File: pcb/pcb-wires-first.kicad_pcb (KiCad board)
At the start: 2 copper layers, 93.7 x 67 mm, 50 parts, among them J10 Conn_01x02, J11 Conn_01x02, J2 Conn_01x02, J5 Conn_01x04, J6 Conn_01x04, J7 Conn_01x04, J9 Conn_01x02, SW1 off-2, SW2 on-2, SW3 on-1, SW4 off-1, SW5 on-3, SW6 off-3, U1 SLG47115V, U2 SLG46826V, U3 R-78C3.3-1.0

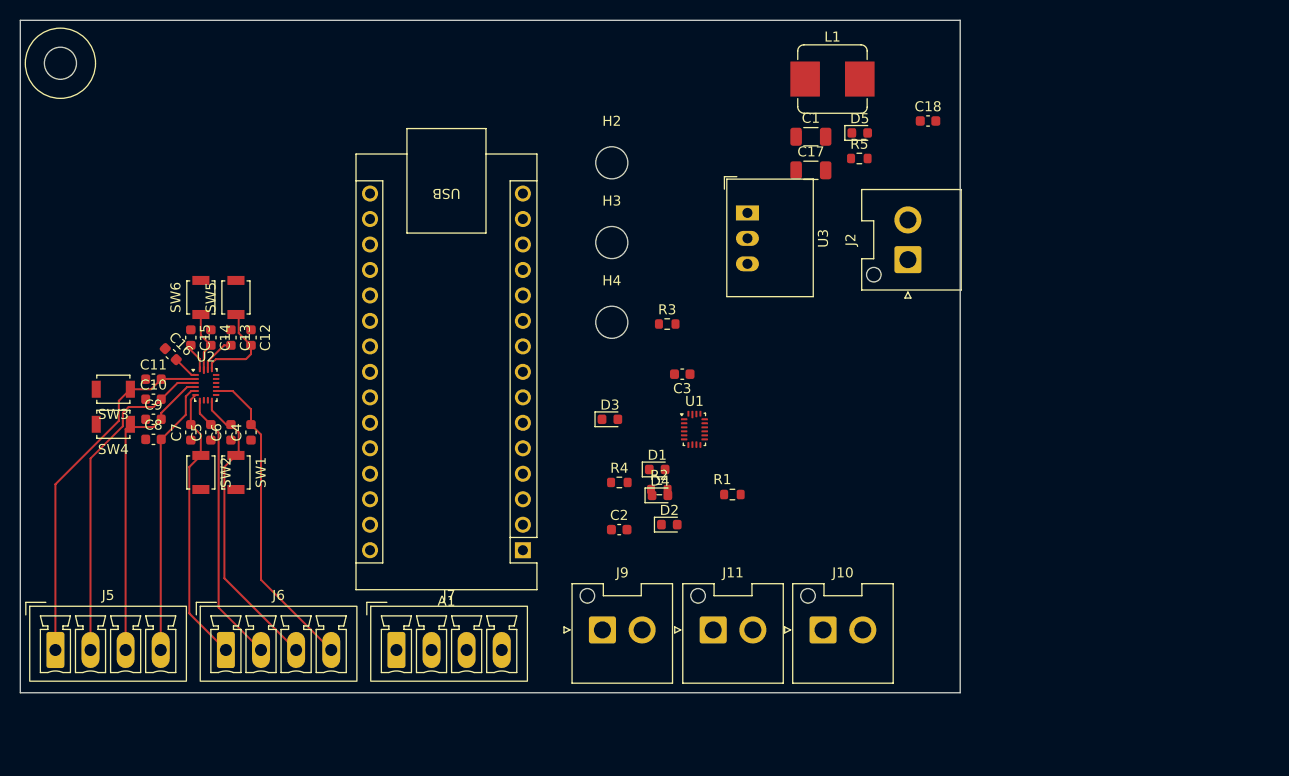
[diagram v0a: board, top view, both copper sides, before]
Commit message: Routing the board.
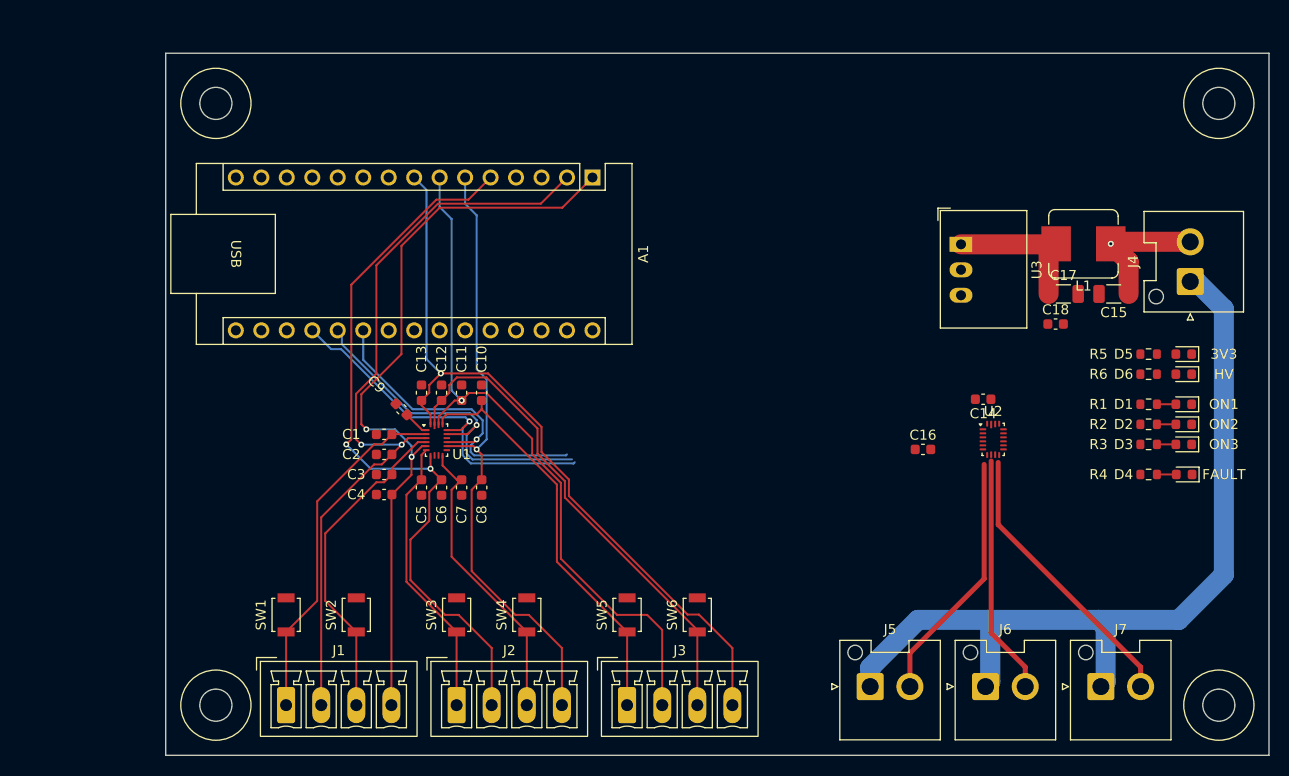
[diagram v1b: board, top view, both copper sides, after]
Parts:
- added D6: HV, Diode_SMD:D_0603_1608Metric, F.Cu at (161.5, 107.0)
- added R6: 6.7k, Resistor_SMD:R_0603_1608Metric, F.Cu at (158.0, 107.0)
- D1: value ON -> ON1
- D2: value FAULT -> ON2
- D3: value ON -> ON3
- D4: value ON -> FAULT
- D5: value FAULT -> 3V3
- R1, R2, R3, R4, R5: value 510 -> 2.2k
- moved H4 71.6 mm to (165.0, 140.0)
- moved H2 60.8 mm to (165.0, 80.0)
- moved H3 60.7 mm to (65.0, 140.0)
- moved SW6 58.8 mm to (113.0, 131.0)
- moved D3 57.3 mm to (161.5, 114.0), turned to 180 degrees
- moved D1 52.9 mm to (161.5, 110.0), turned to 180 degrees
- moved R4 52.8 mm to (158.0, 117.0)
- moved D4 52.3 mm to (161.5, 117.0), turned to 180 degrees
- moved D2 52.3 mm to (161.5, 112.0), turned to 180 degrees
- moved SW5 50.2 mm to (106.0, 131.0)
- moved J7 50.0 mm to (153.2, 138.2)
- moved R3 49.5 mm to (158.0, 114.0)
- moved R2 49.2 mm to (158.0, 112.0)
- moved R1 42.5 mm to (158.0, 110.0)
- moved D5 39.1 mm to (161.5, 105.0), turned to 180 degrees
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- renumbered C11 to C1, C12 to C10, C13 to C11, C14 to C12, C15 to C13, C3 to C14, C17 to C15, C2 to C16, C1 to C17, C10 to C2, C9 to C3, C8 to C4, C7 to C5, C5 to C6, C6 to C7, C4 to C8, C16 to C9, J5 to J1, J6 to J2, J7 to J3, J2 to J4, J11 to J5, J10 to J6, J9 to J7, SW3 to SW1, SW4 to SW2, SW2 to SW3, SW1 to SW4, U2 to U1, U1 to U2
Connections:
- net Net-(A1-A2) renamed switch-1
- A1 pad 19: Net-(A1-A0) -> switch-3
- A1 pad 20: Net-(A1-A1) -> switch-2
- A1 pad 22: unconnected-(A1-A3-Pad22) -> fault
- D2 pad 1: unconnected-(D2-K-Pad1) -> GND
- R2 pad 1: unconnected-(R2-Pad1) -> switch-2
- R3 pad 1: Net-(A1-A1) -> switch-3
- R4 pad 1: Net-(A1-A0) -> switch-3
- R5 pad 1: Net-(U1-GPIO5) -> 3V3
- U1 pad 15: Net-(A1-A1) -> switch-2
- U1 pad 16: Net-(A1-A0) -> switch-3
- U2 pad 14: Net-(A1-A1) -> switch-2
- U2 pad 17: Net-(A1-A0) -> switch-3
- U2 pad 19: Net-(U1-GPIO5) -> fault
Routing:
- net HV-GND: track 0.00 -> 86.0 mm
- net /off-3b: track 2.76 -> 75.4 mm, vias 0 -> 1
- net /on-3b: track 3.78 -> 69.9 mm, vias 0 -> 1
- net /off-1b: track 27.5 -> 76.1 mm, vias 0 -> 2
- net /on-2b: track 27.4 -> 74.6 mm, vias 0 -> 2
- net /on-1b: track 33.5 -> 78.1 mm, vias 0 -> 2
- net /off-3a: track 6.25 -> 50.0 mm
- net switch-3: track 0.00 -> 37.3 mm, vias 0 -> 1
- net switch-2: track 0.00 -> 36.0 mm, vias 0 -> 1
- net switch-1: track 0.00 -> 33.9 mm, vias 0 -> 1
- net /on-3a: track 9.46 -> 41.3 mm
- net /off-2b: track 31.5 -> 62.2 mm, vias 0 -> 1
- net /output-3: track 0.00 -> 28.2 mm
- net /output-1: track 0.00 -> 25.2 mm
- net /output-2: track 0.00 -> 23.9 mm
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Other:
- board size 93.7 x 67 mm -> 110 x 70 mm
